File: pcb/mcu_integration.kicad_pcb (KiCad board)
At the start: 4 copper layers, 70 x 70 mm, 67 parts, among them IC1 TL7660IDGKR, IC2 TL081IDT, IC6 AD844_OPAMP_AL, IC7 FOD814_OPTO_AL, J1 Conn_01x05, J4 Conn_01x02, J5 DM3BT-DSF-PEJS, M1 MountingHole_Pad, M2 MountingHole_Pad, M3 MountingHole_Pad, M4 MountingHole_Pad, U1 STM32F103RBTx, U3 REF192_AL, U6 LM35DM

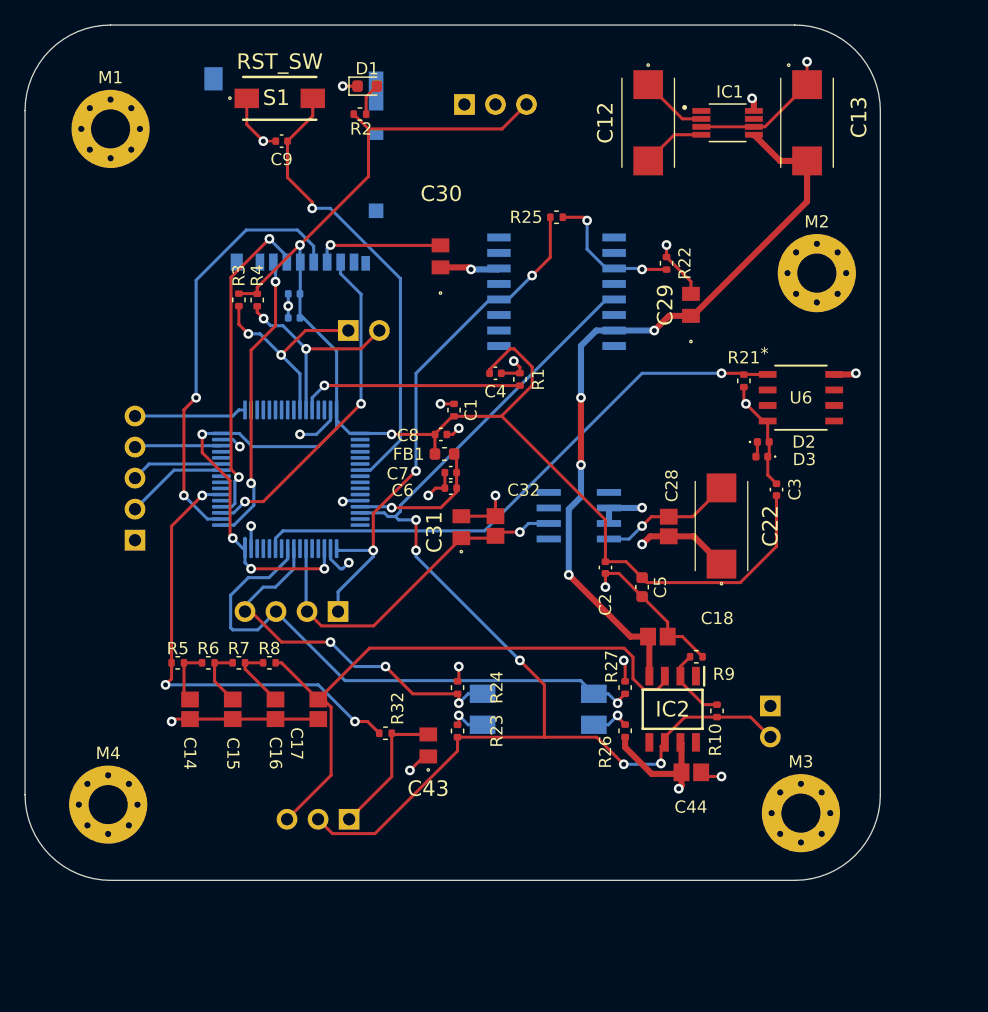
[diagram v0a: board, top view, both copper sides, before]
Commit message: changed footprints and layout
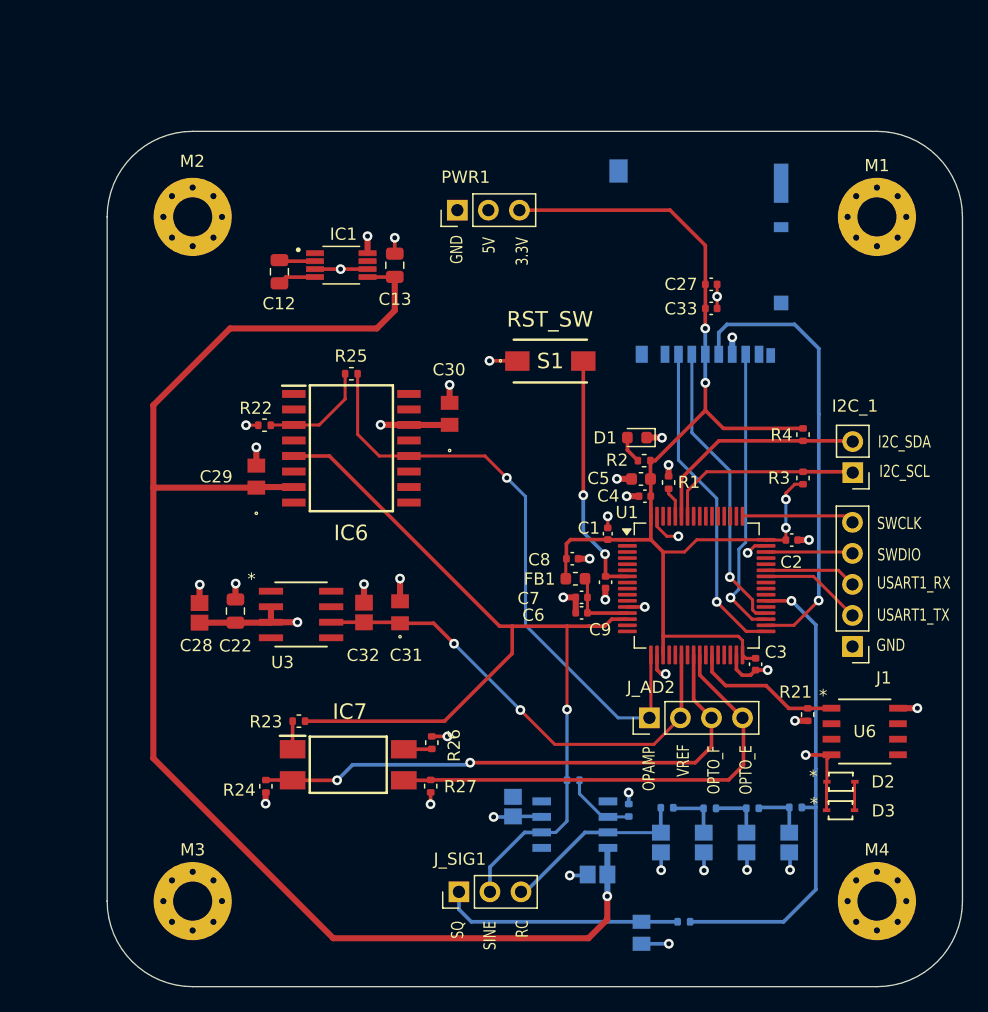
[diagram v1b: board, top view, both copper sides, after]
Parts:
- removed J4: Conn_01x02, Connector_PinHeader_2.54mm:PinHeader_1x02_P2.54mm_Vertical
- C1: footprint Resistor_SMD:R_0402_1005Metric -> Capacitor_SMD:C_0402_1005Metric
- C12, C13, C22: footprint capstone:T495D -> Capacitor_SMD:C_0805_2012Metric
- C14, C15, C16, C17, C18, C43, C44, IC2, M1, M2, M3, M4, R10, R32, R5, R6, R7, R8, R9: moved to B.Cu
- C27, C33, I2C_1, IC6, IC7, J1, J_AD2, J_SIG1, PWR1, U1, U3: moved to F.Cu
- D2, D3: footprint Diode_SMD:D_0402_1005Metric -> capstone:SOD-323_1P7X1P25_ONS
- moved M4 63.4 mm to (173.2, 124.7), turned to 180 degrees
- moved M1 63.1 mm to (173.2, 68.7), turned to 180 degrees
- moved J1 59.4 mm to (171.2, 103.9), turned to 180 degrees
- moved R5 51.9 mm to (166.6, 117.0), turned to 180 degrees
- moved M2 51.3 mm to (117.2, 68.7), turned to 180 degrees
- moved M3 50.3 mm to (117.2, 124.7), turned to 180 degrees
- moved C14 50.2 mm to (166.0, 119.9)
- moved R3 48.4 mm to (167.2, 90.1), turned to 90 degrees
- moved R6 46.1 mm to (163.0, 117.1), turned to 180 degrees
- moved R4 46.0 mm to (167.2, 86.5)
- moved C9 44.8 mm to (151.0, 98.6), turned to 90 degrees
- moved C15 43.4 mm to (162.5, 119.9)
- moved I2C_1 42.9 mm to (171.2, 89.6), turned to 180 degrees
- moved C22 40.4 mm to (120.7, 101.0)
- moved R7 40.3 mm to (159.5, 117.1), turned to 180 degrees
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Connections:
- J_AD2 pad 3: ADC1_IN15_OPTO_E_AL -> ADC1_IN14_OPTO_F_AL
- J_AD2 pad 4: ADC1_IN14_OPTO_F_AL -> ADC1_IN15_OPTO_E_AL
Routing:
- net -5V Output: track 63.0 -> 118.0 mm, vias 4 -> 1
- net 3.3V Output: track 146.8 -> 96.1 mm, vias 6 -> 4
- net GND: track 110.4 -> 64.5 mm, vias 24 -> 37
- net ADC1_IN9_VREG_AL: track 46.8 -> 12.4 mm, vias 1 -> 0
- net RC_OUTPUT: track 50.0 -> 16.0 mm
- net /NRST: track 37.8 -> 20.2 mm, vias 1 -> 2
- net ADC1_IN0_SINE: track 98.2 -> 81.7 mm, vias 5 -> 1
- net /BOOT0: track 18.4 -> 2.48 mm, vias 1 -> 0
- net ADC1_IN14_OPTO_F_AL: track 30.6 -> 45.7 mm, vias 3 -> 2
- net ADC1_IN6_VREF_AL: track 29.0 -> 38.9 mm, vias 1 -> 2
- net Net-(J_SIG1-Pin_1): track 11.5 -> 19.8 mm
- net ADC1_IN3_OPAMP_AL: track 43.4 -> 50.6 mm, vias 3 -> 1
- net ADC1_IN15_OPTO_E_AL: track 45.9 -> 39.0 mm, vias 1 -> 0
- net +5V: track 29.8 -> 23.3 mm
- net Net-(U1-VDDA): track 11.6 -> 6.15 mm, vias 1 -> 0
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- added copper zone on In1.Cu, net +5V
- added copper zone on In2.Cu, net GND
- removed copper zone on In2.Cu, net +5V
- removed copper zone on In1.Cu, net GND
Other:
- board text added: "3.3V"
- board text added: "5V"
- board text added: "GND"
- board text added: "I2C_SCL"
- board text added: "I2C_SDA"
- board text added: "OPAMP"
- board text added: "OPTO_E"
- board text added: "OPTO_F"
- board text added: "RC"
- board text added: "SINE"
- board text added: "SQ"
- board text added: "VREF"
